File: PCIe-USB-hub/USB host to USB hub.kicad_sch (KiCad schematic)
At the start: 1 part

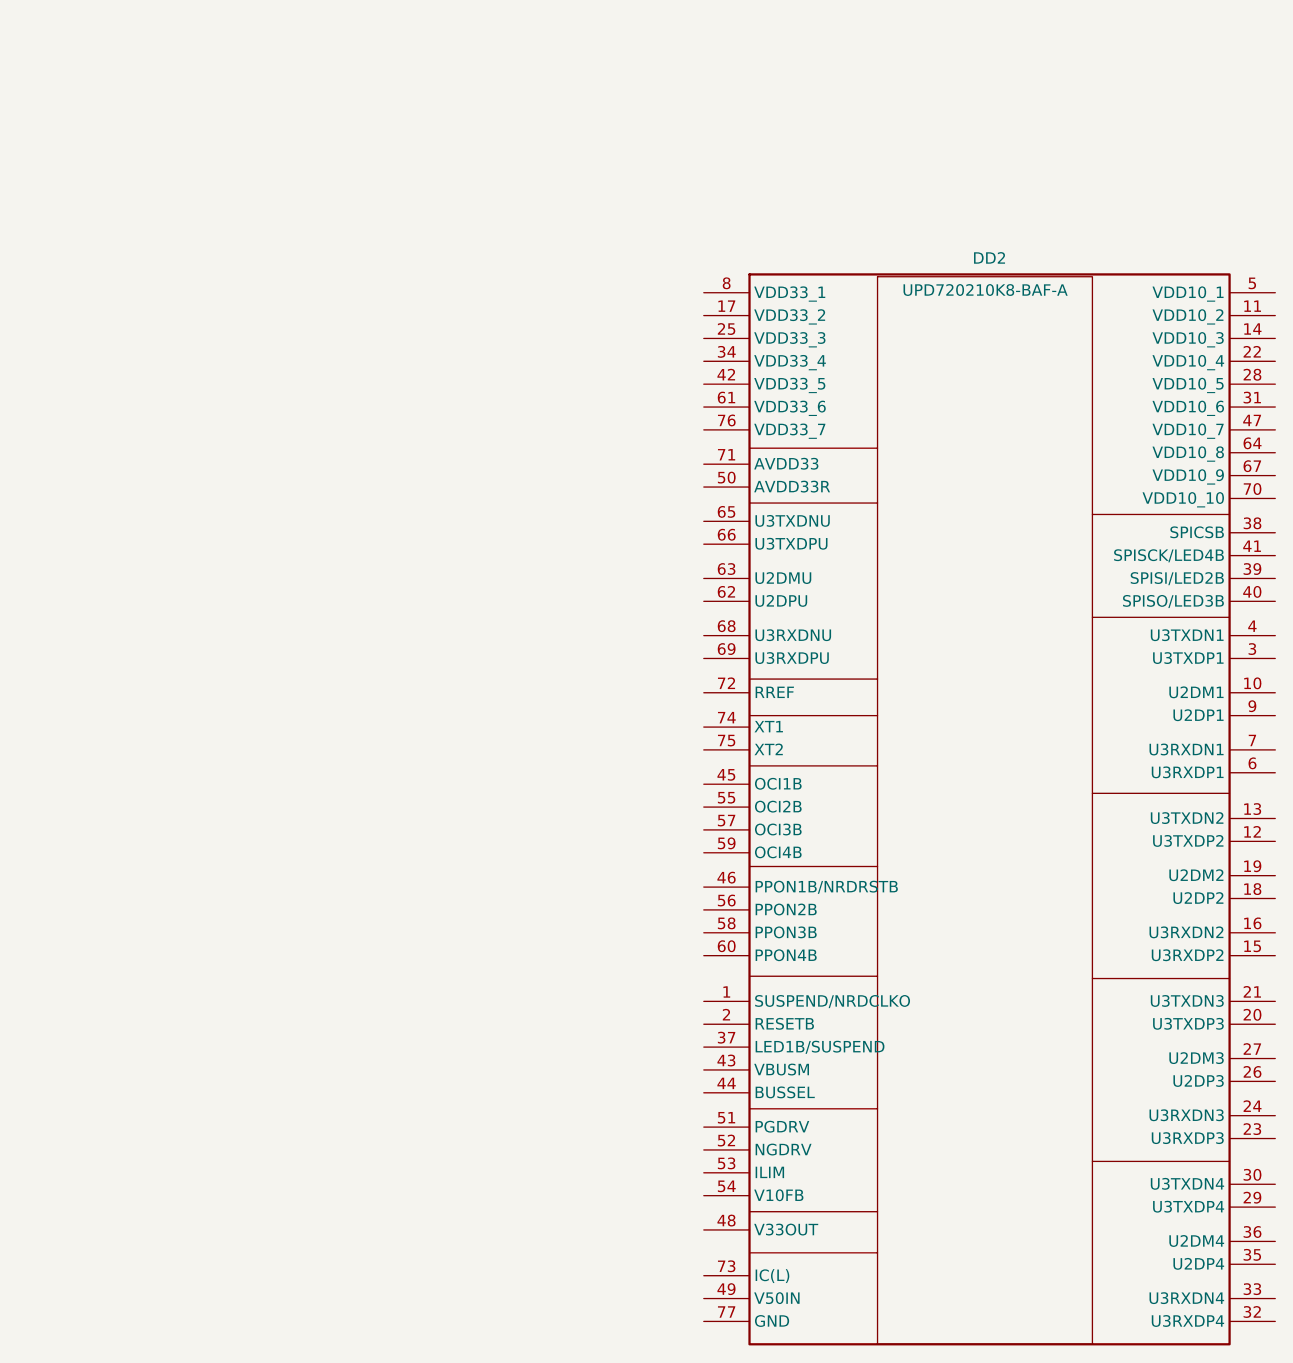
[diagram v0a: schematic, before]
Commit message: Частично добавил компоненты
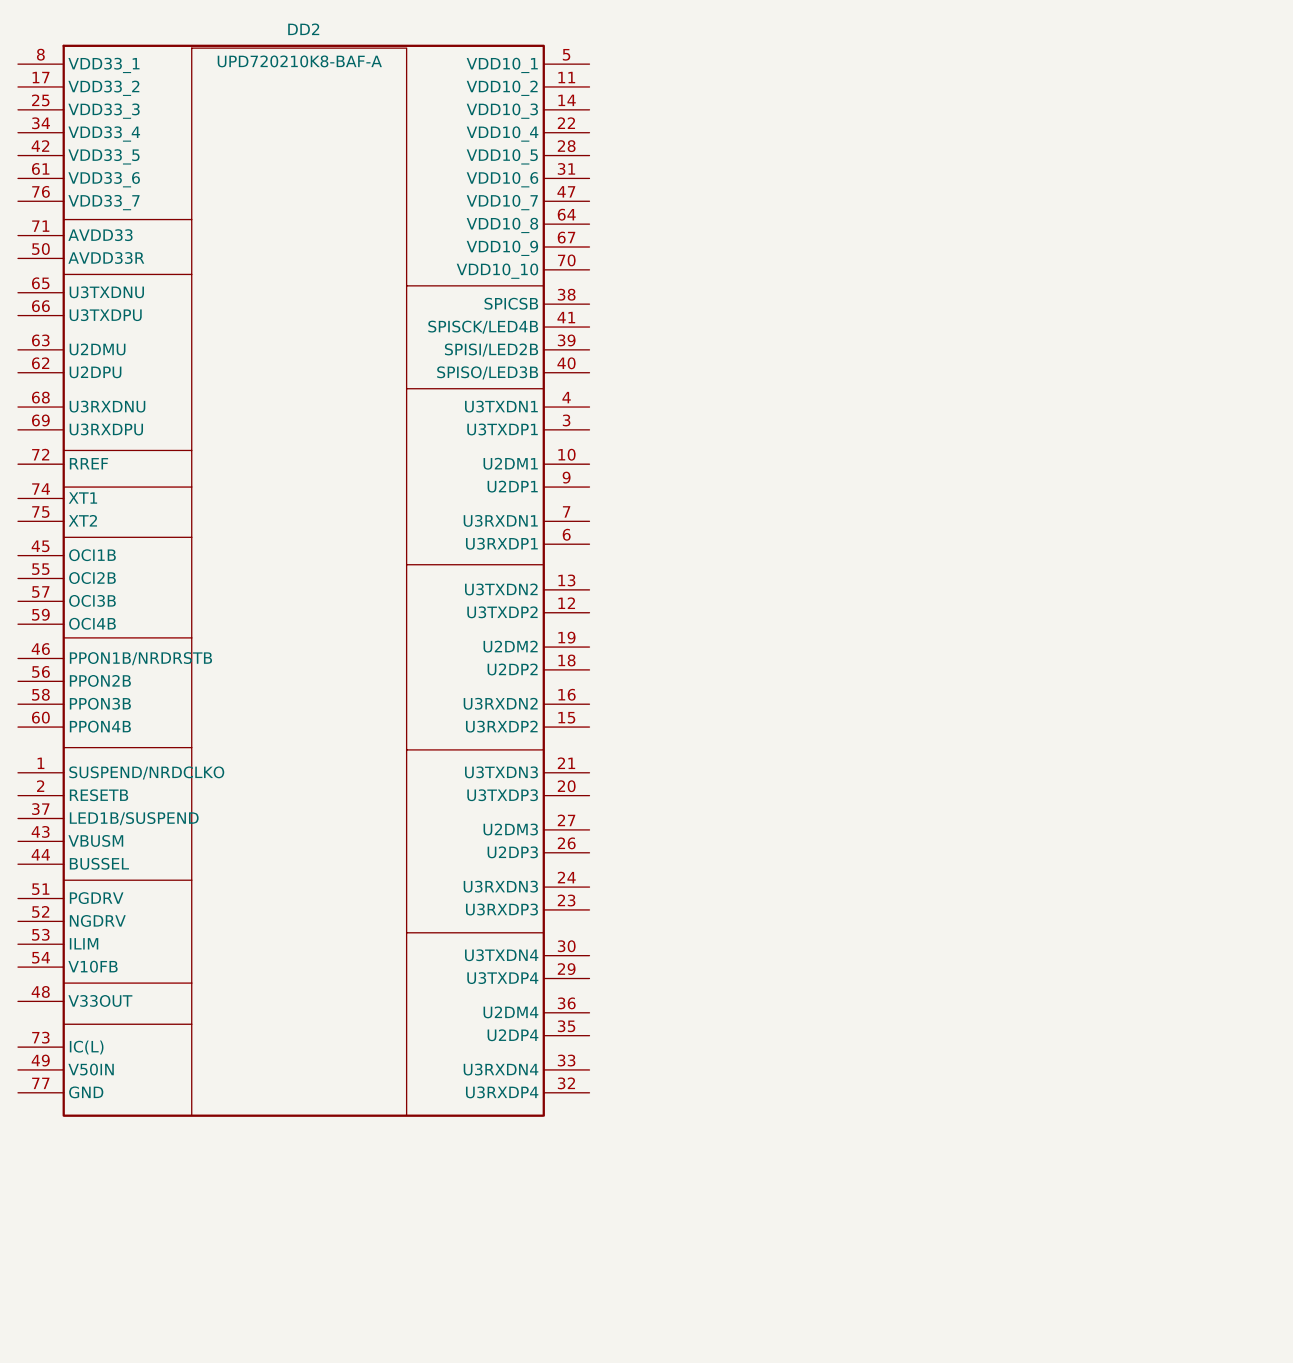
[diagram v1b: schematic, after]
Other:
- moved on the sheet: DD2
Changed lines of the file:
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@@
 	(symbol
 		(lib_id "UPD720210K8-BAF-A:UPD720210K8-BAF-A")
-		(at 172.72 135.89 0)
+		(at 96.52 110.49 0)
 		(unit 1)
 		(exclude_from_sim no)
@@
 		(dnp no)
 		(property "Reference" "DD2"
-			(at 204.47 83.82 0)
+			(at 128.27 58.42 0)
 			(effects
 				(font
@@
 		)
 		(property "Value" "UPD720210K8-BAF-A"
-			(at 203.962 87.376 0)
+			(at 127.762 61.976 0)
 			(effects
 				(font
@@
 		)
 		(property "Footprint" "Package_DFN_QFN:QFN-76-1EP_9x9mm_P0.4mm_EP5.81x6.31mm"
-			(at 210.312 218.44 0)
+			(at 134.112 193.04 0)
 			(effects
 				(font
@@
 		)
 		(property "Datasheet" "https://media.digikey.com/pdf/Data%20Sheets/~No%20Display/Renesas%20PDFs/uPD720210_DS.pdf"
-			(at 232.41 318.11 0)
+			(at 156.21 292.71 0)
 			(effects
 				(font
@@
 		)
 		(property "Description" "The PD720210 is a 4-Port USB 3.0 hub controller, which complies with Universal Serial Bus 3.0 Specification and is 100% compatible with Renesas industry-standard host controllers. The controller provides four downstream USB ports. Each of these ports supports is fully backward compatible with all previous versions of USB, LS (Low-Speed) / FS (Full-Speed) / HS (High-Speed) / SS (SuperSpeed) operation.uPD720210 comes in a 76-pin QFN package. A few of the benefits that this device provides to system designer"
-			(at 171.704 220.726 0)
+			(at 95.504 195.326 0)
 			(effects
 				(font
@@
 		)
 		(property "Height" "0.9"
-			(at 232.41 518.11 0)
+			(at 156.21 492.71 0)
 			(effects
 				(font
@@
 		)
 		(property "Manufacturer_Name" "Renesas Electronics"
-			(at 232.41 618.11 0)
+			(at 156.21 592.71 0)
 			(effects
 				(font
@@
 		)
 		(property "Manufacturer_Part_Number" "UPD720210K8-BAF-A"
-			(at 232.41 718.11 0)
+			(at 156.21 692.71 0)
 			(effects
 				(font
@@
 		)
 		(property "Mouser Part Number" "968-UPD720210K8BAFA"
-			(at 232.41 818.11 0)
+			(at 156.21 792.71 0)
 			(effects
 				(font
@@
 		)
 		(property "Mouser Price/Stock" "https://www.mouser.co.uk/ProductDetail/Renesas-Electronics/UPD720210K8-BAF-A?qs=ZVKuL1Ob8AsZ2EpJ%252BfgVCw%3D%3D"
-			(at 232.41 918.11 0)
+			(at 156.21 892.71 0)
 			(effects
 				(font
@@
 		)
 		(property "Arrow Part Number" "UPD720210K8-BAF-A"
-			(at 232.41 1018.11 0)
+			(at 156.21 992.71 0)
 			(effects
 				(font
@@
 		)
 		(property "Arrow Price/Stock" "https://www.arrow.com/en/products/upd720210k8-baf-a/renesas-electronics"
-			(at 232.41 1118.11 0)
+			(at 156.21 1092.71 0)
 			(effects
 				(font
